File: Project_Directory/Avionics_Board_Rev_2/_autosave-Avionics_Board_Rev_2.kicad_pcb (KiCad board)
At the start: 2 copper layers, 60 x 120 mm, 80 parts, among them J1 Battery, J10 PWM_1, J11 PWM_2, J12 PWM_3, J13 I2C, J14 UART, J15 Conn_Coaxial, J2 ARM, J3 PYRO_1, J4 PYRO_1, J5 PYRO_1, J6 PYRO_1, J7 PWM_4, J8 PWM_5, J9 PWM_6, Q1 Drive_MOS, Q2 Drive_MOS, Q3 Drive_MOS, Q4 Drive_MOS, U1 Teensy4.1, U10 GSM, U11 AP2127K-3.3, U2 LoRa - RFM95-W/PW, U3 ADXL, U4 ADS1115IDGS, U5 AMS1117-3.3, U6 GPS, U7 GY-91, U8 AMS1117-5.0

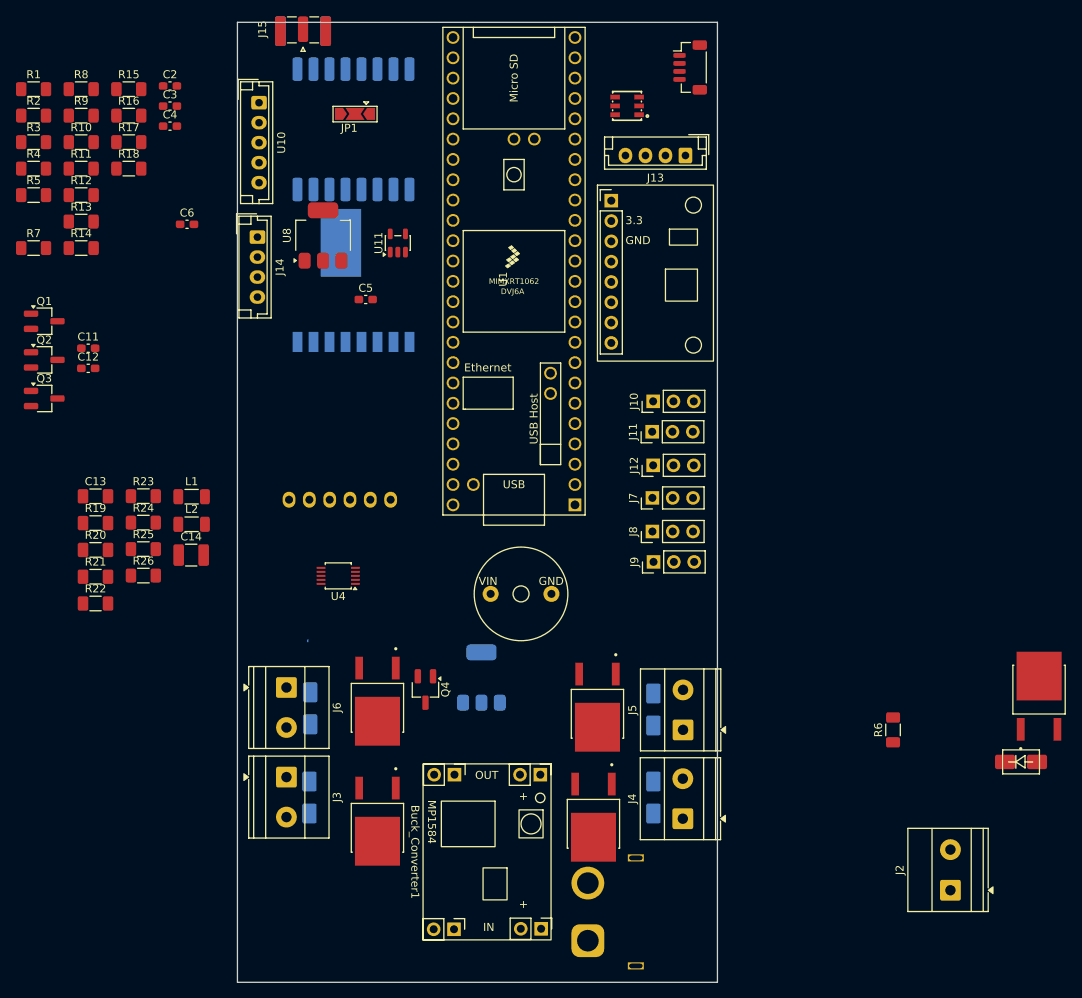
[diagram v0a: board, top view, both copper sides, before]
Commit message: temp
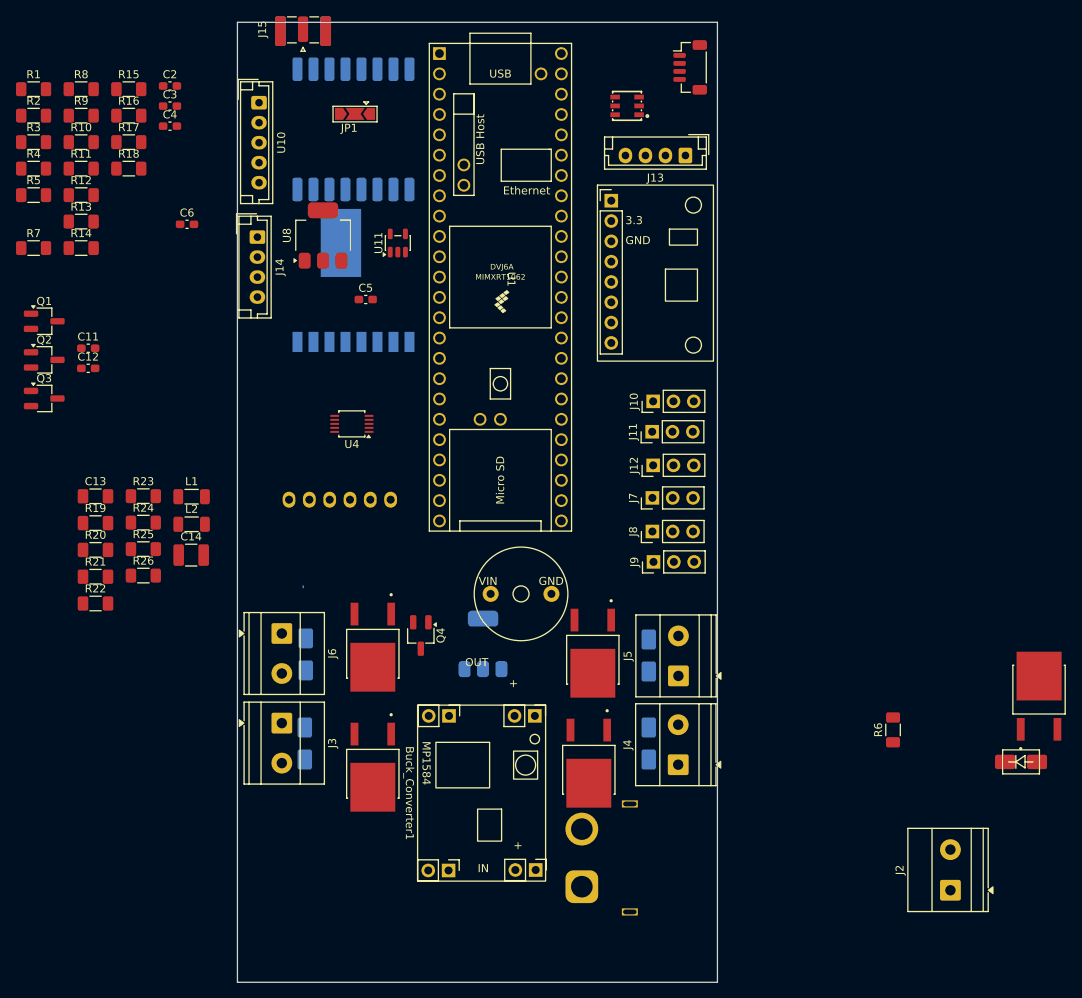
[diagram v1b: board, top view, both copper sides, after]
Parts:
- moved U4 19.1 mm to (98.8, 104.0)
- moved Buck_Converter1 7.38 mm to (115.0, 150.1)
- moved J1 6.79 mm to (127.5, 161.8)
- moved J4 6.77 mm to (139.6, 146.6)
- moved C1 6.77 mm to (101.4, 146.9)
- moved C10 6.77 mm to (101.4, 131.9)
- moved D1 6.77 mm to (92.9, 143.9)
- moved D5 6.77 mm to (93.0, 132.8)
- moved J3 6.77 mm to (90.0, 141.3)
- moved J6 6.77 mm to (90.0, 130.2)
- moved Q4 6.77 mm to (107.4, 130.4)
- moved C8 6.77 mm to (128.4, 146.4)
- moved C9 6.77 mm to (128.9, 132.6)
- moved D3 6.77 mm to (135.9, 143.9)
- moved D4 6.77 mm to (135.9, 132.9)
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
